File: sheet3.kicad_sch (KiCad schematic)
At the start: 18 parts, among them J7 Screw_Terminal_01x02, J8 Screw_Terminal_01x02, U6 MAX3485, U7 MAX3485

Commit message: Autosave
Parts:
- D3, D4: MPN (none) -> SM712
- R29, R30, R31, R32, R33, R35, R36, R37, R38, R39: MPN (none) -> 0402WGJ0103TCE
- R34, R40: MPN (none) -> 0402WGF1200TCE
- U6, U7: MPN (none) -> MAX3485ESA(UMW)
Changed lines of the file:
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@@
+			)
+		)
+		(property "MPN" "0402WGJ0103TCE"
+			(at 49.53 34.29 0)
+			(hide yes)
+			(show_name no)
+			(do_not_autoplace no)
+			(effects
+				(font
+					(size 1.27 1.27)
+				)
 			)
 		)
@@
 			)
 		)
+		(property "MPN" "MAX3485ESA(UMW)"
+			(at 80.01 49.53 0)
+			(hide yes)
+			(show_name no)
+			(do_not_autoplace no)
+			(effects
+				(font
+					(size 1.27 1.27)
+				)
+			)
+		)
 		(pin "2"
 		)
@@
 			)
 		)
+		(property "MPN" ""
+			(at 163.83 43.18 0)
+			(hide yes)
+			(show_name no)
+			(do_not_autoplace no)
+			(effects
+				(font
+					(size 1.27 1.27)
+				)
+			)
+		)
 		(pin "1"
 		)
@@
 			)
 		)
+		(property "MPN" "0402WGF1200TCE"
+			(at 137.16 97.79 0)
+			(hide yes)
+			(show_name no)
+			(do_not_autoplace no)
+			(effects
+				(font
+					(size 1.27 1.27)
+				)
+			)
+		)
 		(pin "2"
 		)
@@
 			)
 		)
+		(property "MPN" "0402WGJ0103TCE"
+			(at 96.52 106.68 0)
+			(hide yes)
+			(show_name no)
+			(do_not_autoplace no)
+			(effects
+				(font
+					(size 1.27 1.27)
+				)
+			)
+		)
 		(pin "2"
 		)
@@
 			)
 		)
+		(property "MPN" "0402WGJ0103TCE"
+			(at 57.15 34.29 0)
+			(hide yes)
+			(show_name no)
+			(do_not_autoplace no)
+			(effects
+				(font
+					(size 1.27 1.27)
+				)
+			)
+		)
 		(pin "2"
 		)
@@
 			)
 		)
+		(property "MPN" "0402WGJ0103TCE"
+			(at 49.53 87.63 0)
+			(hide yes)
+			(show_name no)
+			(do_not_autoplace no)
+			(effects
+				(font
+					(size 1.27 1.27)
+				)
+			)
+		)
 		(pin "2"
 		)
@@
 			)
 		)
+		(property "MPN" "0402WGJ0103TCE"
+			(at 96.52 34.29 0)
+			(hide yes)
+			(show_name no)
+			(do_not_autoplace no)
+			(effects
+				(font
+					(size 1.27 1.27)
+				)
+			)
+		)
 		(pin "2"
 		)
@@
 			)
 		)
+		(property "MPN" "SM712"
+			(at 121.92 97.79 90)
+			(hide yes)
+			(show_name no)
+			(do_not_autoplace no)
+			(effects
+				(font
+					(size 1.27 1.27)
+				)
+			)
+		)
 		(pin "1"
 		)
@@
 			)
 		)
+		(property "MPN" "0402WGJ0103TCE"
+			(at 96.52 53.34 0)
+			(hide yes)
+			(show_name no)
+			(do_not_autoplace no)
+			(effects
+				(font
+					(size 1.27 1.27)
+				)
+			)
+		)
 		(pin "2"
 		)
@@
 			)
 		)
+		(property "MPN" "0402WGJ0103TCE"
+			(at 57.15 87.63 0)
+			(hide yes)
+			(show_name no)
+			(do_not_autoplace no)
+			(effects
+				(font
+					(size 1.27 1.27)
+				)
+			)
+		)
 		(pin "2"
 		)
@@
 			)
 		)
+		(property "MPN" "MAX3485ESA(UMW)"
+			(at 80.01 102.87 0)
+			(hide yes)
+			(show_name no)
+			(do_not_autoplace no)
+			(effects
+				(font
+					(size 1.27 1.27)
+				)
+			)
+		)
 		(pin "2"
 		)
@@
 			)
 		)
+		(property "MPN" ""
+			(at 163.83 96.52 0)
+			(hide yes)
+			(show_name no)
+			(do_not_autoplace no)
+			(effects
+				(font
+					(size 1.27 1.27)
+				)
+			)
+		)
 		(pin "1"
 		)
@@
 			)
 		)
+		(property "MPN" "0402WGJ0103TCE"
+			(at 41.91 34.29 0)
+			(hide yes)
+			(show_name no)
+			(do_not_autoplace no)
+			(effects
+				(font
+					(size 1.27 1.27)
+				)
+			)
+		)
 		(pin "1"
 		)
@@
 			)
 		)
+		(property "MPN" "0402WGF1200TCE"
+			(at 137.16 44.45 0)
+			(hide yes)
+			(show_name no)
+			(do_not_autoplace no)
+			(effects
+				(font
+					(size 1.27 1.27)
+				)
+			)
+		)
 		(pin "2"
 		)
@@
 			)
 		)
+		(property "MPN" "0402WGJ0103TCE"
+			(at 96.52 87.63 0)
+			(hide yes)
+			(show_name no)
+			(do_not_autoplace no)
+			(effects
+				(font
+					(size 1.27 1.27)
+				)
+			)
+		)
 		(pin "2"
 		)
@@
 			)
 		)
+		(property "MPN" "SM712"
+			(at 121.92 44.45 90)
+			(hide yes)
+			(show_name no)
+			(do_not_autoplace no)
+			(effects
+				(font
+					(size 1.27 1.27)
+				)
+			)
+		)
 		(pin "1"
 		)
@@
 			(at 41.91 87.63 0)
 			(hide yes)
+			(show_name no)
+			(do_not_autoplace no)
+			(effects
+				(font
+					(size 1.27 1.27)
+				)
+			)
+		)
+		(property "MPN" "0402WGJ0103TCE"
+			(at 41.91 87.63 0)
+			(hide yes)

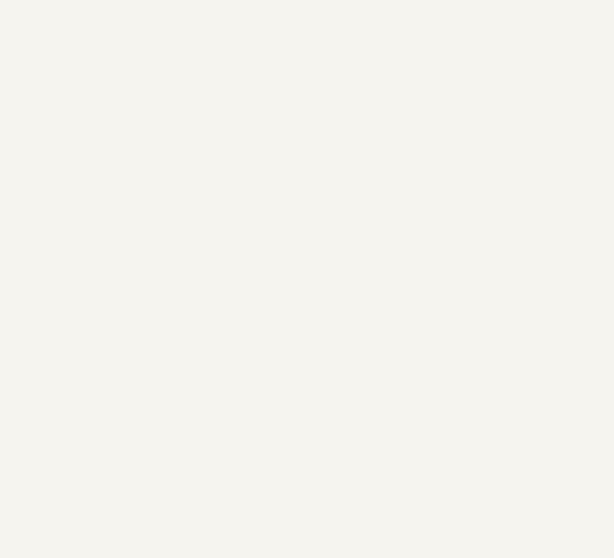
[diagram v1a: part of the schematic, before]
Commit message: Autosave
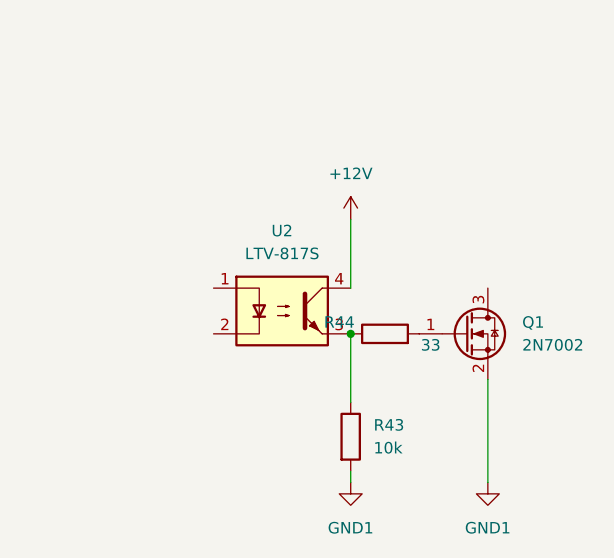
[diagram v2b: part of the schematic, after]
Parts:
- added Q1: 2N7002, Package_TO_SOT_SMD:SOT-23, symbol Transistor_FET:2N7002
- added R43: 10k, Resistor_SMD:R_0402_1005Metric, symbol Device:R
- added R44: 33, Resistor_SMD:R_0402_1005Metric, symbol Device:R
- added U2: LTV-817S, Package_DIP:SMDIP-4_W9.53mm, symbol Isolator:LTV-817S
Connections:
- new net: R43.1, R44.1, U2.3
- new net: Q1.1 (G), R44.2
- new net +12V: U2.4
- new net GND1: Q1.2 (S), R43.2
